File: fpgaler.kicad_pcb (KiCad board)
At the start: 4 copper layers, 188 x 165.2 mm, 286 parts, among them J1 USB_C_Receptacle_USB2.0, J3 JTAG, J4 FTDI_RST, J5 VGA, J6 DB9 Expander, J7 DB9 Expander, Q1 BC817, SW1 RotaryEncoder_Switch, SW2 RotaryEncoder_Switch, SW3 K1, SW4 K2, SW5 PROGRAMN, SW6 K3, SW7 FPGA GSRN, SW8 K4, U1 TLV62569DRL, U10 XC6206PxxxMR, U11 IS62WV51216BLL-55TLI, U2 TLV62569DRL, U3 NCP115-2.5, U5 93LC56BT-I/OT, U6 FT2232HL, U7 CAT24C128, U8 LFE5U-25F-8MG285C, U9 W25Q128JVP, X1 27MHz, Y1 7M-12.000MAAJ

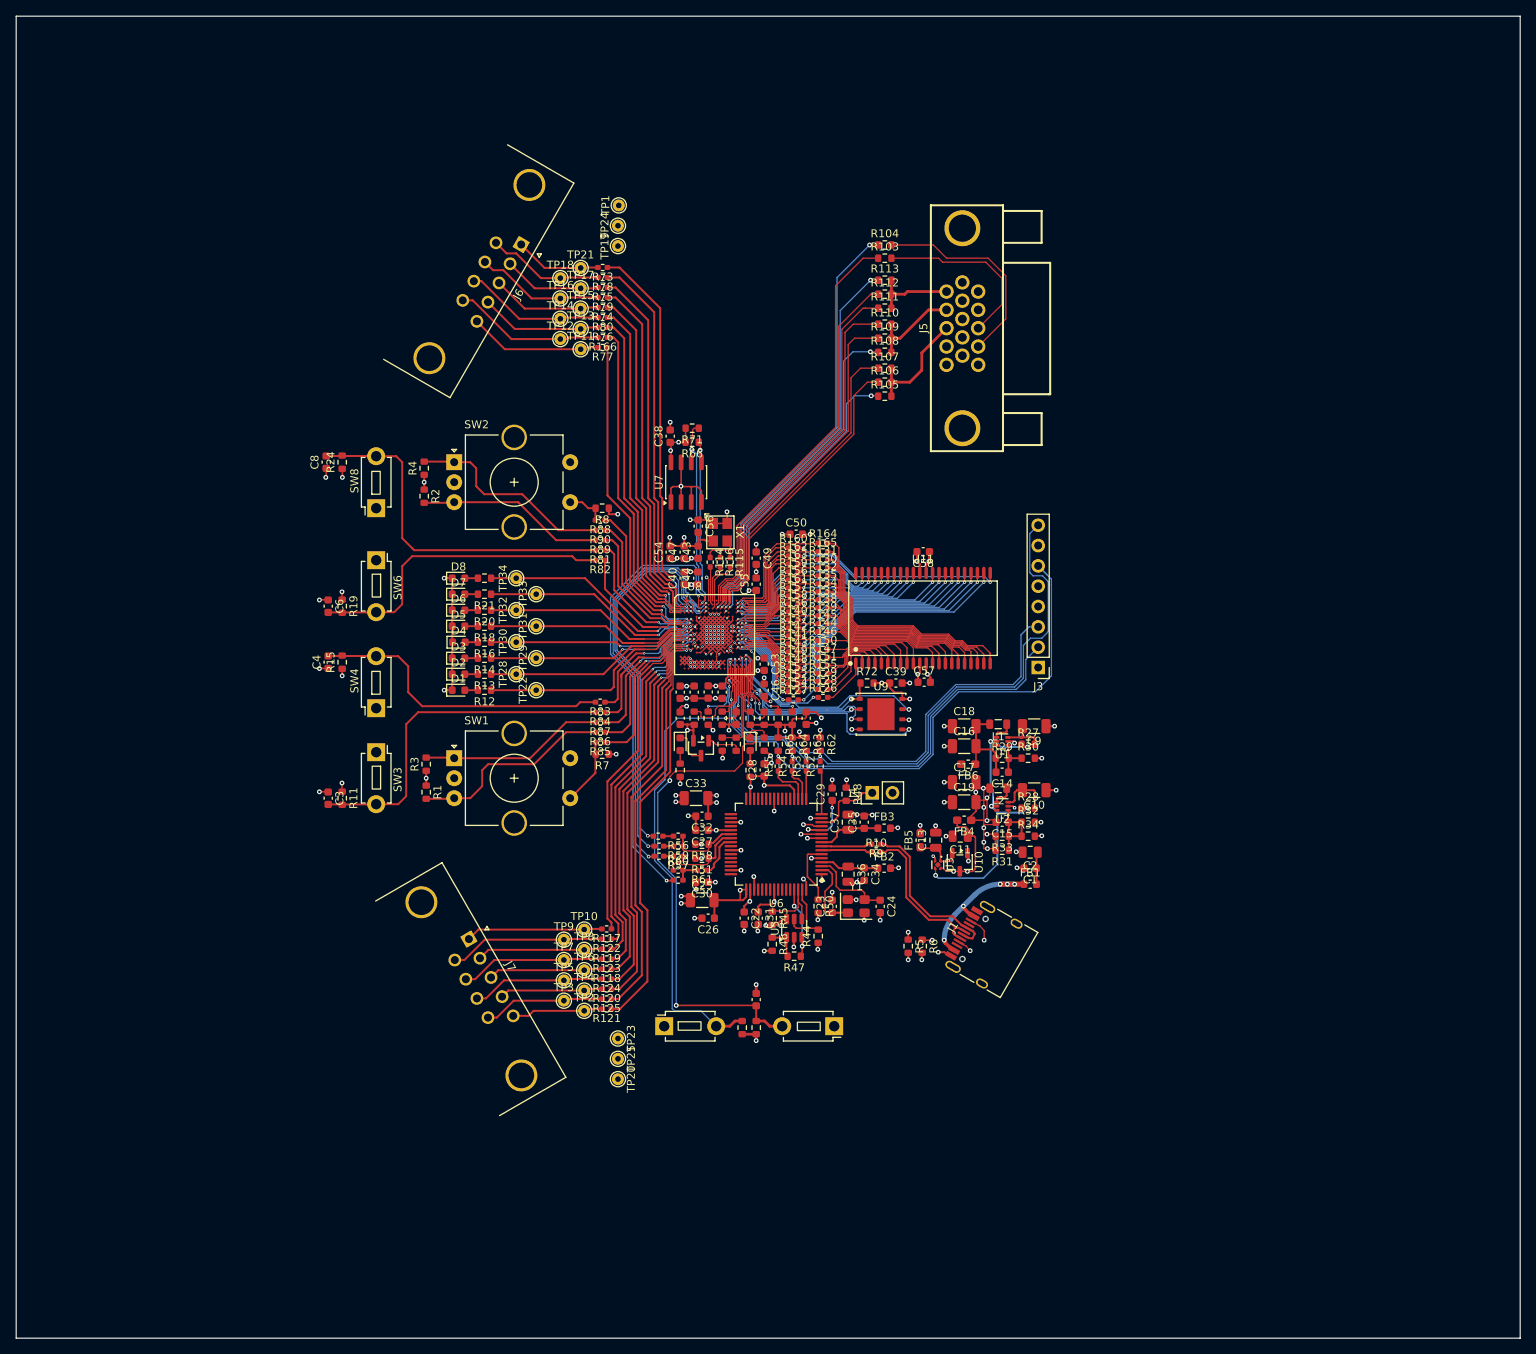
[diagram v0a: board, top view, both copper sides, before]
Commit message: Continue routing
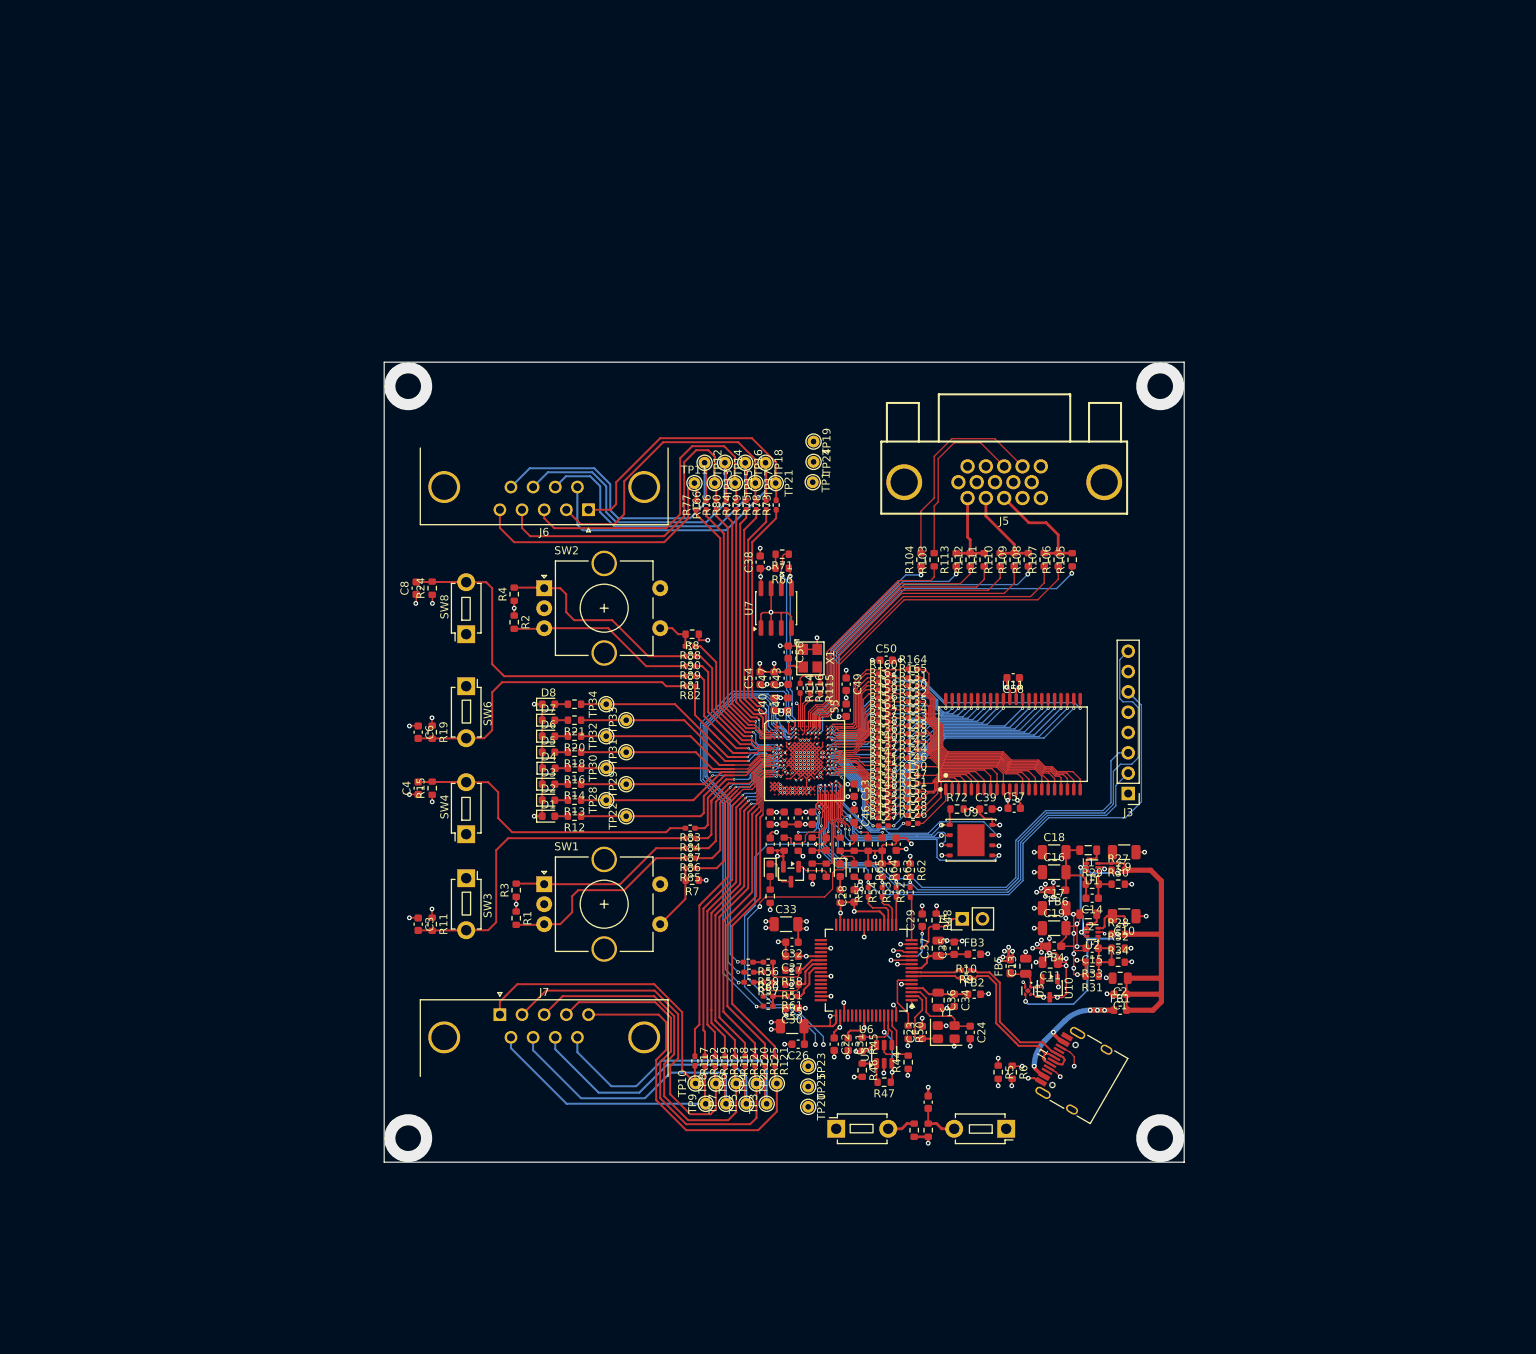
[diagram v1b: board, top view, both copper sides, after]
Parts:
- moved TP1 42.3 mm to (133.6, 60.0), turned to -90 degrees
- moved R104 39.6 mm to (147.1, 69.7), turned to 90 degrees
- moved TP24 38.3 mm to (133.7, 57.5), turned to -90 degrees
- moved R103 38.2 mm to (148.7, 69.7), turned to 90 degrees
- moved R73 36.8 mm to (129.0, 62.9), turned to 90 degrees
- moved TP21 36.3 mm to (128.9, 60.1), turned to -90 degrees
- moved R113 36.1 mm to (151.5, 69.7), turned to 90 degrees
- moved R78 35.0 mm to (127.8, 62.9), turned to 90 degrees
- moved R112 34.9 mm to (153.2, 69.7), turned to 90 degrees
- moved TP19 34.6 mm to (133.7, 54.9), turned to -90 degrees
- moved TP18 34.5 mm to (127.7, 57.6), turned to -90 degrees
- moved J6 34.2 mm to (105.5, 63.4), turned to 180 degrees
- moved R111 33.8 mm to (155.0, 69.7), turned to 90 degrees
- moved R75 33.3 mm to (126.5, 62.9), turned to 90 degrees
- moved R110 32.8 mm to (157.0, 69.7), turned to 90 degrees
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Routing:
- net GND: track 1108.4 -> 896.1 mm, vias 119 -> 123
- net +5V: track 16.6 -> 54.9 mm
- net /P0_DB4: track 12.9 -> 45.4 mm
- net /P0_DB5: track 11.4 -> 43.8 mm
- net /P0_DB2: track 14.3 -> 45.3 mm
- net /P0_DB3: track 15.7 -> 44.9 mm
- net /FPGA/VGA_VSYNC: track 54.8 -> 28.4 mm
- net /P1_DB2: track 13.7 -> 39.8 mm
- net /P1_DB4: track 15.2 -> 41.1 mm
- net /P1_DB3: track 12.3 -> 37.1 mm
- net /P1_DB6: track 14.6 -> 38.8 mm
- net /P1_DB1: track 10.8 -> 34.8 mm
- net /P1_DB7: track 16.1 -> 39.5 mm
- net /FPGA/VGA_HSYNC: track 53.3 -> 30.0 mm
- net /P0_DB9: track 15.2 -> 38.4 mm
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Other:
- board size 188 x 165.2 mm -> 100 x 100 mm
